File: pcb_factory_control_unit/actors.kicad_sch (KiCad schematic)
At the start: 79 parts, among them J17 Elevator, J18 Sorter, J19 Vacuum Pump, J20 Bus-Servo, J21 Cylinder Valve, J22 RoArm, J23 Conveyor, J24 Compressor, J25 Vacuum Valve, J26 Disturbance1, J27 Disturbance2, Q3 AO3400, Q4 AO3400, Q5 AO3400, Q6 AO3400, Q7 AO3400, Q8 AO3400, U10 TMC2209, U11 74AHCT125, U9 TMC2209

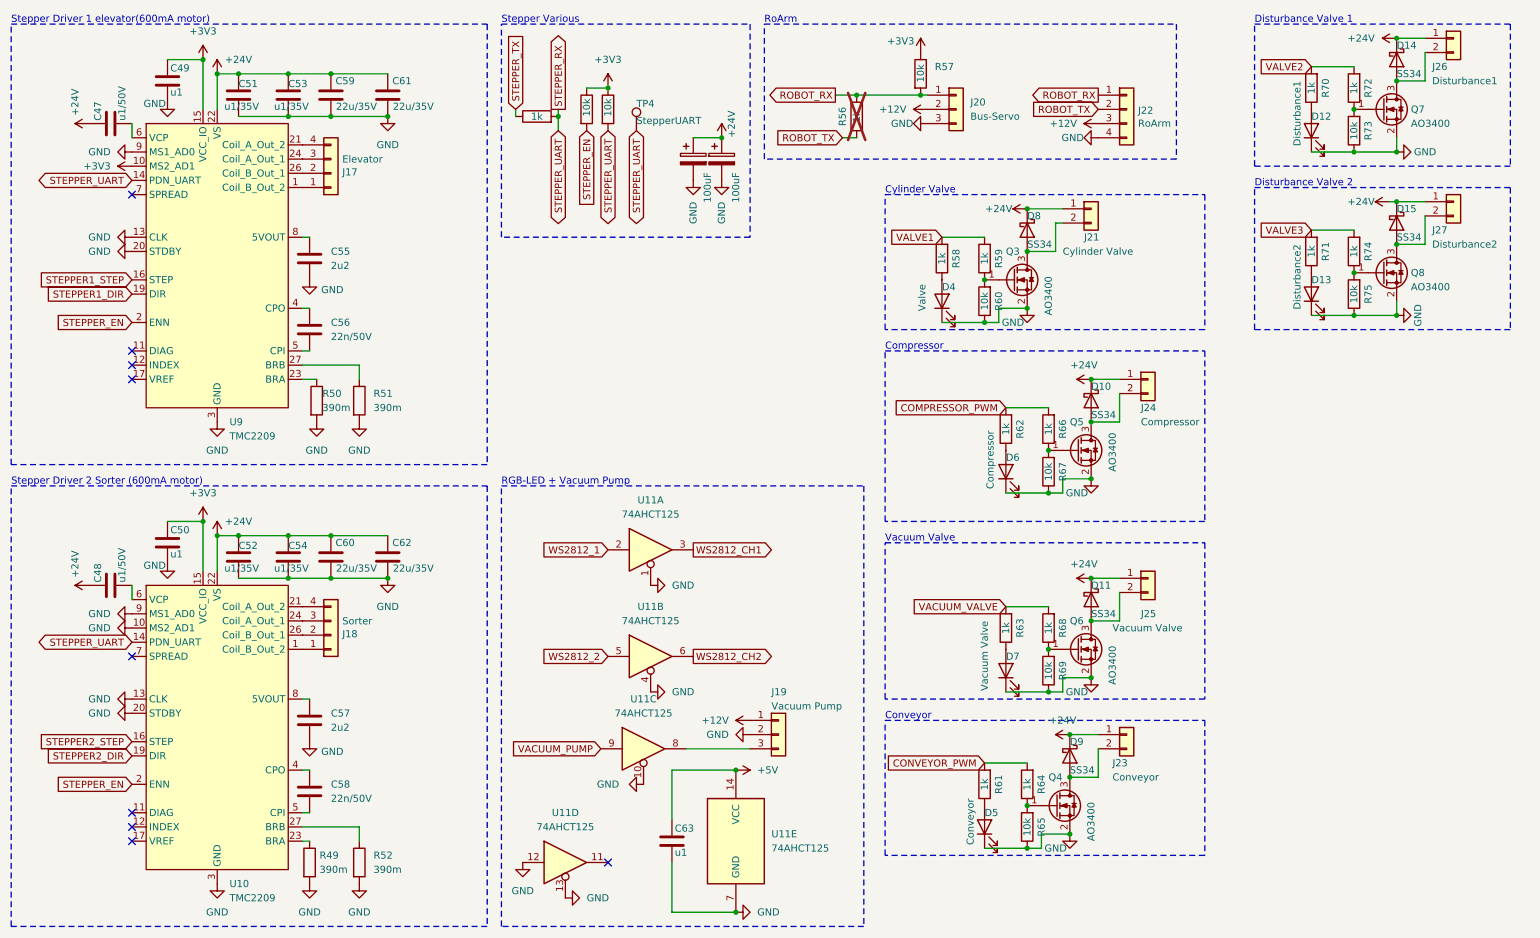
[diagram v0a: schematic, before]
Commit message: PCB WIP
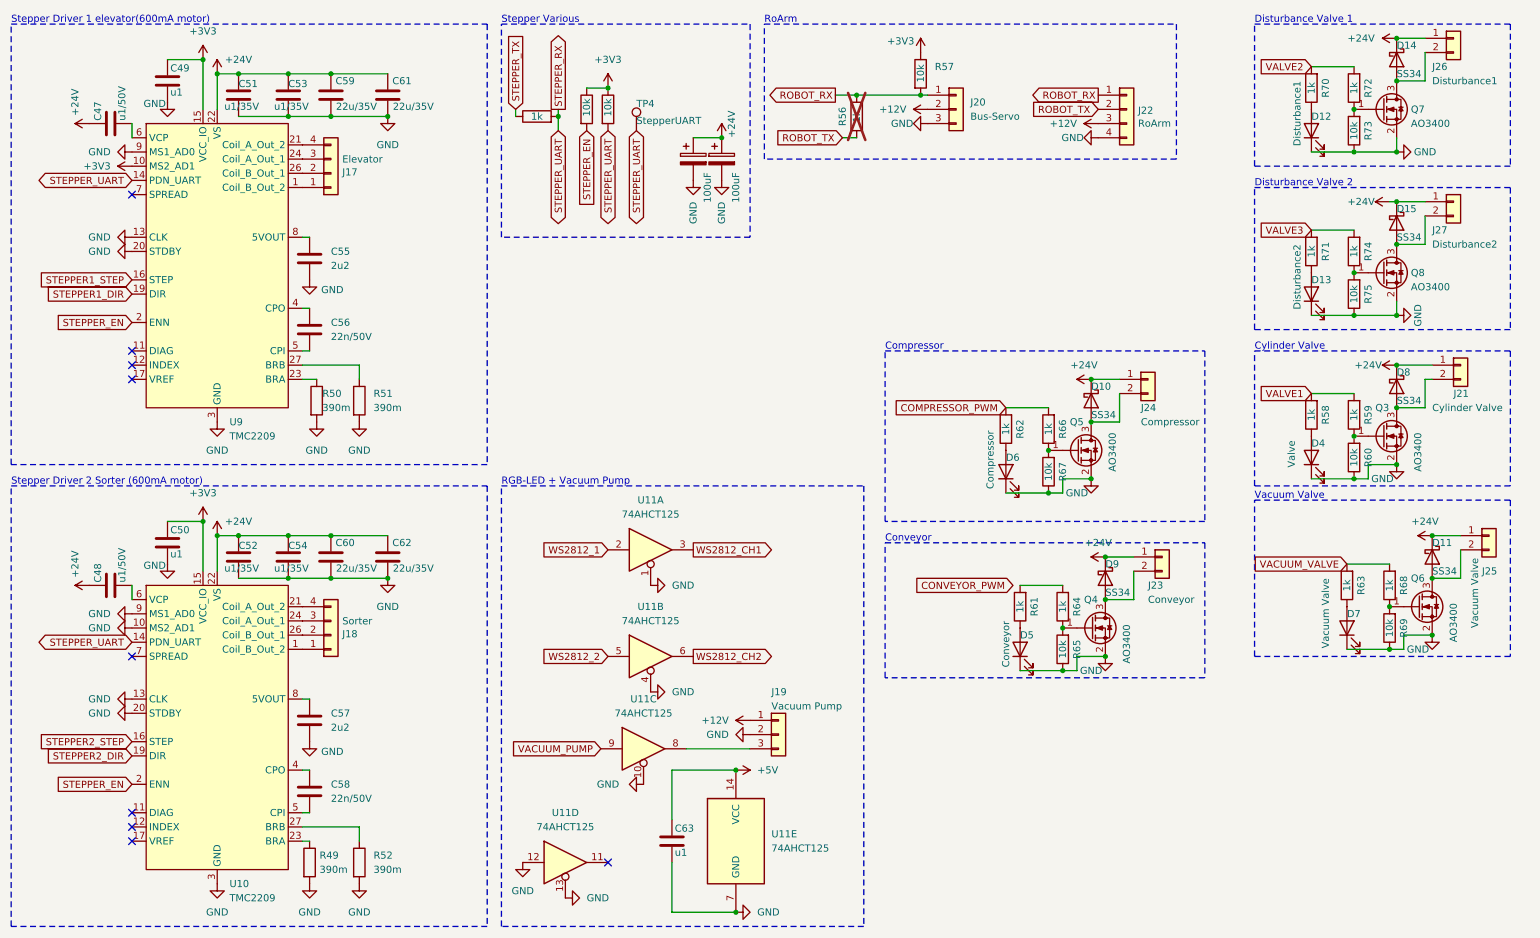
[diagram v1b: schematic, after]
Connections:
- net CONVEYOR_PWM: no longer R61.2, R64.2
- new net: R61.2, R64.2
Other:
- moved on the sheet: D11, D4, D5, D7, D8, D9, J21, J23, J25, Q3, Q4, Q6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
